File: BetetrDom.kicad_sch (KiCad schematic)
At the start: 10 parts, among them J1 XT60PW-M, J2 Raspberry_Pi_2_3

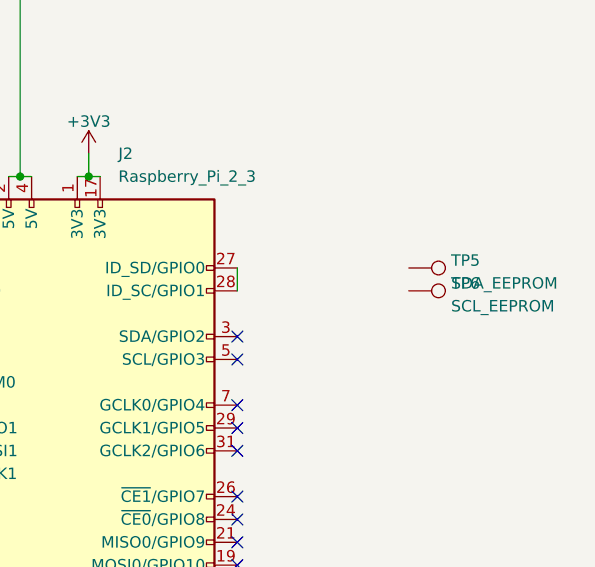
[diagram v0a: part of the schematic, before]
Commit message: UPDATE
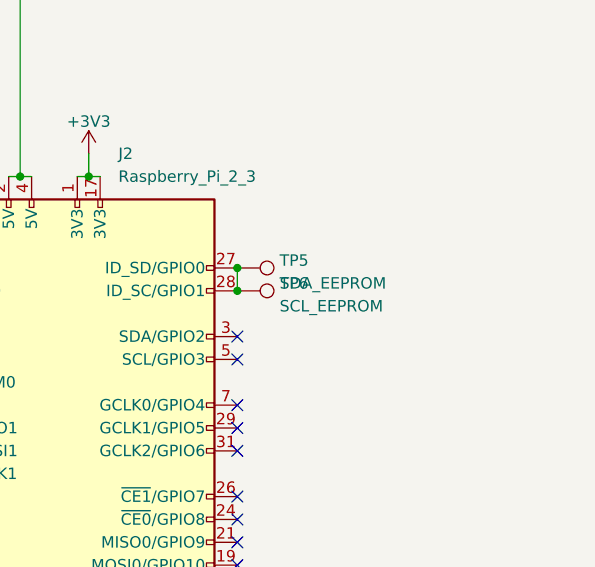
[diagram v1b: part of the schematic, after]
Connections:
- net at J2.27 (ID_SD/GPIO0), J2.28 (ID_SC/GPIO1): now also TP5.1, TP6.1
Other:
- moved on the sheet: TP5, TP6
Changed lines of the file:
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@@
 	(paper "A4")
+	(junction
+		(at 194.31 77.47)
+		(diameter 0)
+		(color 0 0 0 0)
+	)
 	(junction
 		(at 179.07 133.35)
@@
 	(junction
 		(at 41.91 59.69)
+		(diameter 0)
+		(color 0 0 0 0)
+	)
+	(junction
+		(at 194.31 80.01)
 		(diameter 0)
 		(color 0 0 0 0)
@@
 	(symbol
 		(lib_id "Connector:TestPoint")
-		(at 213.36 80.01 270)
+		(at 194.31 80.01 270)
 		(unit 1)
 		(exclude_from_sim no)
@@
 		(fields_autoplaced yes)
 		(property "Reference" "TP6"
-			(at 218.059 79.1753 90)
+			(at 199.009 79.1753 90)
 			(effects
 				(font
@@
 		)
 		(property "Value" "SCL_EEPROM"
-			(at 218.059 81.7122 90)
+			(at 199.009 81.7122 90)
 			(effects
 				(font
@@
 		)
 		(property "Footprint" "TestPoint:TestPoint_Pad_1.5x1.5mm"
-			(at 213.36 85.09 0)
+			(at 194.31 85.09 0)
 			(effects
 				(font
@@
 		)
 		(property "Datasheet" "~"
-			(at 213.36 85.09 0)
+			(at 194.31 85.09 0)
 			(effects
 				(font
@@
 		)
 		(property "Description" ""
-			(at 213.36 80.01 0)
+			(at 194.31 80.01 0)
 			(effects
 				(font
@@
 	(symbol
 		(lib_id "Connector:TestPoint")
-		(at 213.36 77.47 270)
+		(at 194.31 77.47 270)
 		(unit 1)
 		(exclude_from_sim no)
@@
 		(fields_autoplaced yes)
 		(property "Reference" "TP5"
-			(at 218.059 76.6353 90)
+			(at 199.009 76.6353 90)
 			(effects
 				(font
@@
 		)
 		(property "Value" "SDA_EEPROM"
-			(at 218.059 79.1722 90)
+			(at 199.009 79.1722 90)
 			(effects
 				(font
@@
 		)
 		(property "Footprint" "TestPoint:TestPoint_Pad_1.5x1.5mm"
-			(at 213.36 82.55 0)
+			(at 194.31 82.55 0)
 			(effects
 				(font
@@
 		)
 		(property "Datasheet" "~"
-			(at 213.36 82.55 0)
+			(at 194.31 82.55 0)
 			(effects
 				(font
@@
 		)
 		(property "Description" ""
-			(at 213.36 77.47 0)
-			(effects
-				(font
+			(at 194.31 77.47 0)
+			(effects
+				(font

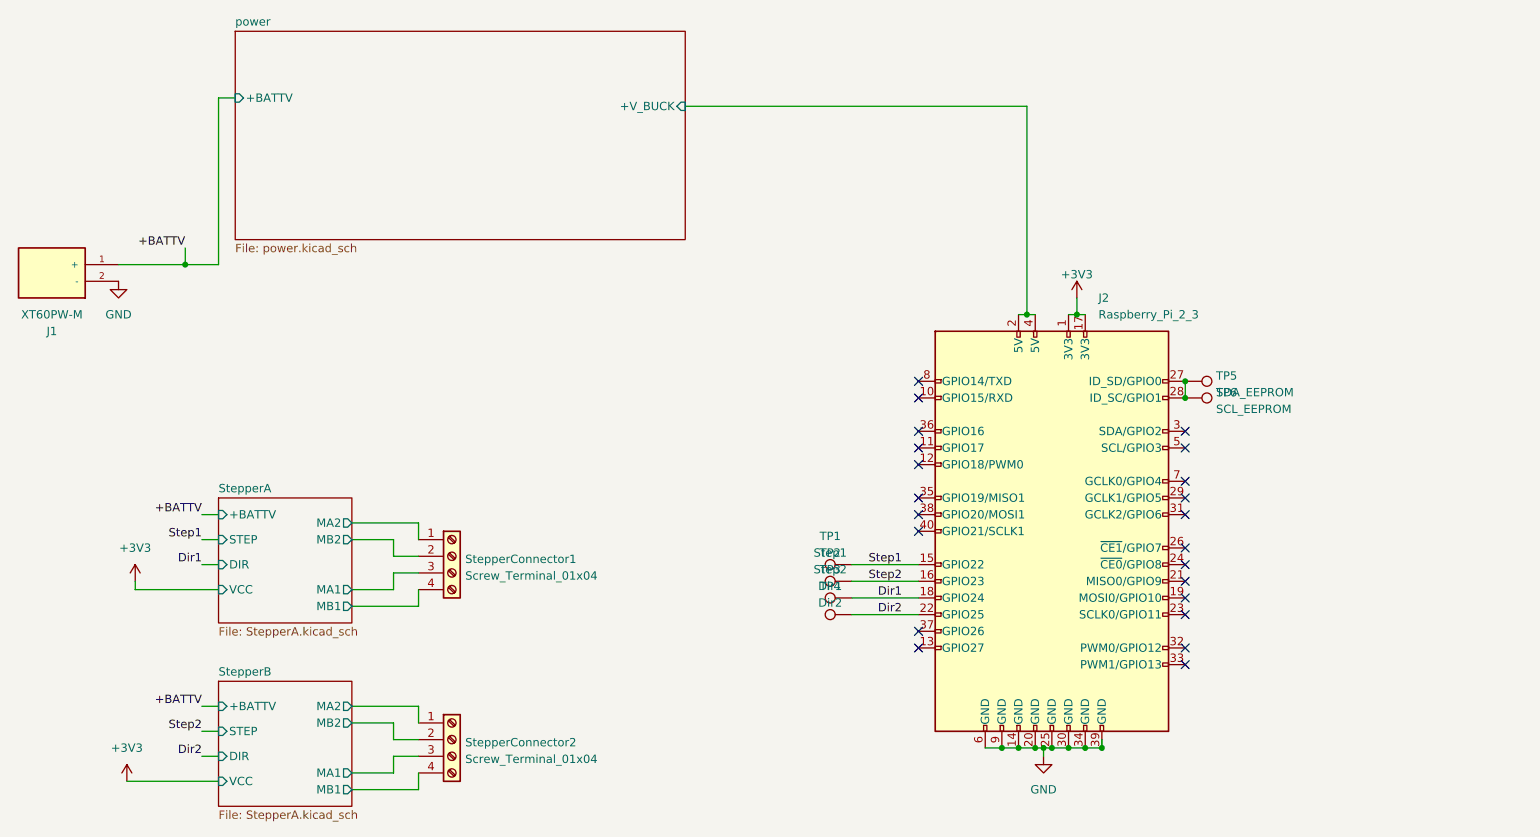
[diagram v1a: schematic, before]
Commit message: finished pcb layouts, ready for check p sure
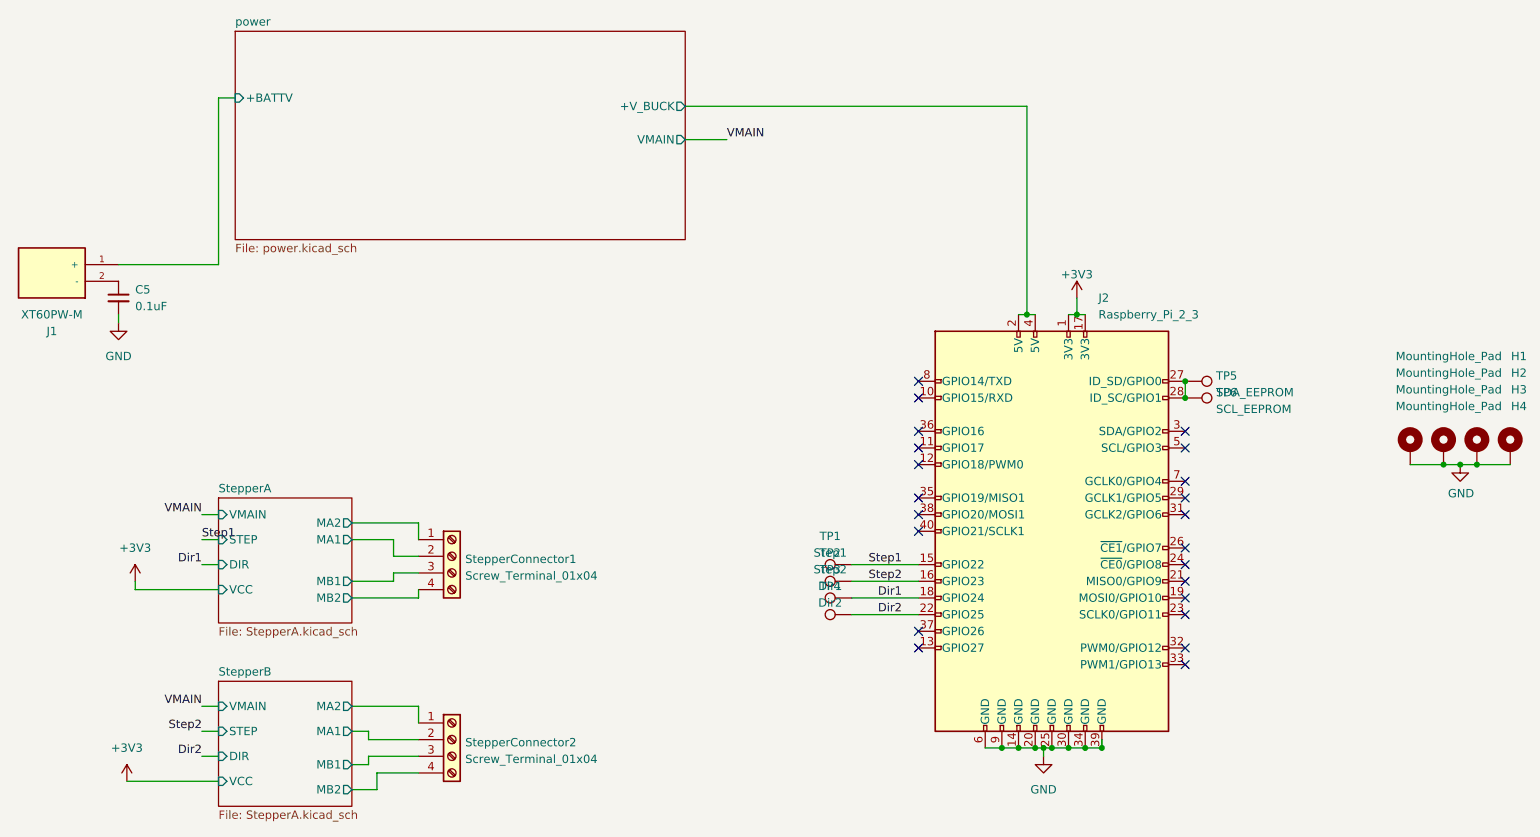
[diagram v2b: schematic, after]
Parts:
- added C5: 0.1uF, Capacitor_SMD:C_0402_1005Metric, symbol Device:C_Small
- added H1, H2, H3, H4: MountingHole_Pad, MountingHole:MountingHole_3.2mm_M3_DIN965_Pad, symbol Mechanical:MountingHole_Pad
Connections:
- net GND: now also C5.2, H1.1, H2.1, H3.1, H4.1; no longer J1.2 (-)
- net StepperA/MA1: now also StepperConnector1.2 (Pin_2); no longer StepperConnector1.3 (Pin_3)
- net StepperA/MB1: now also StepperConnector1.3 (Pin_3); no longer StepperConnector1.4 (Pin_4)
- net StepperA/MB2: now also StepperConnector1.4 (Pin_4); no longer StepperConnector1.2 (Pin_2)
- net StepperB/MA1: now also StepperConnector2.2 (Pin_2); no longer StepperConnector2.3 (Pin_3)
- net StepperB/MB1: now also StepperConnector2.3 (Pin_3); no longer StepperConnector2.4 (Pin_4)
- net StepperB/MB2: now also StepperConnector2.4 (Pin_4); no longer StepperConnector2.2 (Pin_2)
- net +BATTV renamed power/+BATTV
- new net: C5.1, J1.2 (-)
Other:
- sheet StepperA ports: added VMAIN; removed +BATTV
- sheet StepperB ports: added VMAIN; removed +BATTV
- sheet power ports: added VMAIN; removed none

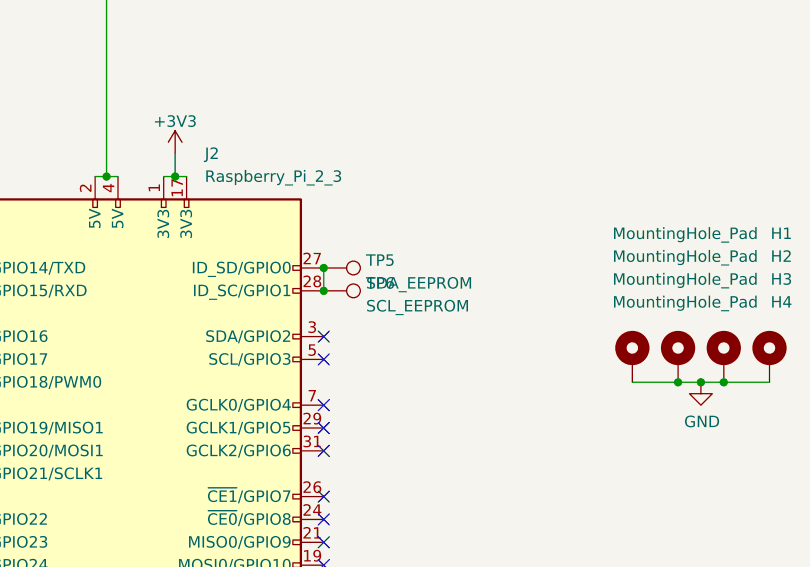
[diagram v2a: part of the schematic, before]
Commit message: update
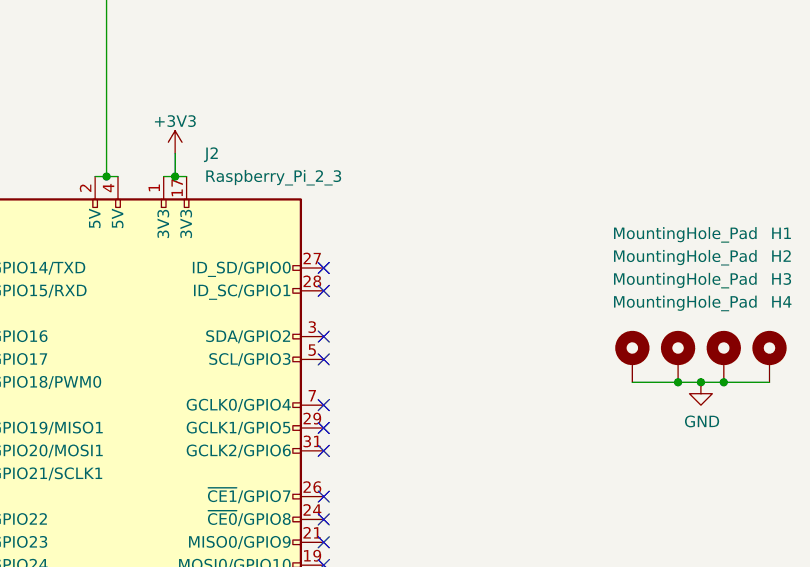
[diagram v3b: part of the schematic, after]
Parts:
- removed TP5: SDA_EEPROM, TestPoint:TestPoint_Pad_1.5x1.5mm, symbol Connector:TestPoint
- removed TP6: SCL_EEPROM, TestPoint:TestPoint_Pad_1.5x1.5mm, symbol Connector:TestPoint
- StepperConnector1, StepperConnector2: footprint TerminalBlock_TE-Connectivity:TerminalBlock_TE_282834-4_1x04_P2.54mm_Horizontal -> Connector_Molex:Molex_Nano-Fit_105313-xx04_1x04_P2.50mm_Horizontal
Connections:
- net at J2.27 (ID_SD/GPIO0): no longer J2.28 (ID_SC/GPIO1)
- no-connect marks 22 -> 24
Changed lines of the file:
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@@
 	(paper "A4")
-	(junction
-		(at 194.31 77.47)
-		(diameter 0)
-		(color 0 0 0 0)
-	)
 	(junction
 		(at 233.68 90.17)
@@
 	)
 	(junction
-		(at 194.31 80.01)
-		(diameter 0)
-		(color 0 0 0 0)
-	)
-	(junction
 		(at 166.37 133.35)
 		(diameter 0)
@@
 	)
 	(no_connect
+		(at 194.31 80.01)
+	)
+	(no_connect
+		(at 194.31 77.47)
+	)
+	(no_connect
 		(at 194.31 92.71)
 	)
@@
 		(pts
 			(xy 69.85 130.81) (xy 67.31 130.81)
-		)
-		(stroke
-			(width 0)
-			(type default)
-		)
-	)
-	(wire
-		(pts
-			(xy 194.31 77.47) (xy 194.31 80.01)
 		)
 		(stroke
@@
 	)
 	(symbol
-		(lib_id "Connector:TestPoint")
-		(at 194.31 80.01 270)
-		(unit 1)
-		(exclude_from_sim no)
-		(in_bom yes)
-		(on_board yes)
-		(dnp no)
-		(fields_autoplaced yes)
-		(property "Reference" "TP6"
-			(at 199.009 79.1753 90)
-			(effects
-				(font
-					(size 1.27 1.27)
-				)
-				(justify left)
-			)
-		)
-		(property "Value" "SCL_EEPROM"
-			(at 199.009 81.7122 90)
-			(effects
-				(font
-					(size 1.27 1.27)
-				)
-				(justify left)
-			)
-		)
-		(property "Footprint" "TestPoint:TestPoint_Pad_1.5x1.5mm"
-			(at 194.31 85.09 0)
-			(effects
-				(font
-					(size 1.27 1.27)
-				)
-				(hide yes)
-			)
-		)
-		(property "Datasheet" "~"
-			(at 194.31 85.09 0)
-			(effects
-				(font
-					(size 1.27 1.27)
-				)
-				(hide yes)
-			)
-		)
-		(property "Description" ""
-			(at 194.31 80.01 0)
-			(effects
-				(font
-					(size 1.27 1.27)
-				)
-				(hide yes)
-			)
-		)
-		(pin "1"
-		)
-		(instances
-			(project "BetetrDom"
-				(path "/3d73b00f-865e-402b-88ef-ae22e0a8ba36"
-					(reference "TP6")
-					(unit 1)
-				)
-			)
-		)
-	)
-	(symbol
 		(lib_id "Connector:Screw_Terminal_01x04")
 		(at 82.55 104.14 0)
@@
 			)
 		)
-		(property "Footprint" "TerminalBlock_TE-Connectivity:TerminalBlock_TE_282834-4_1x04_P2.54mm_Horizontal"
+		(property "Footprint" "Connector_Molex:Molex_Nano-Fit_105313-xx04_1x04_P2.50mm_Horizontal"
 			(at 82.55 104.14 0)
 			(effects
@@
 			)
 		)
-		(property "Footprint" "TerminalBlock_TE-Connectivity:TerminalBlock_TE_282834-4_1x04_P2.54mm_Horizontal"
+		(property "Footprint" "Connector_Molex:Molex_Nano-Fit_105313-xx04_1x04_P2.50mm_Horizontal"
 			(at 82.55 132.08 0)
 			(effects
@@
 					(unit 1)
 				)
-			)
-		)
-	)
-	(symbol
-		(lib_id "Connector:TestPoint")
-		(at 194.31 77.47 270)
-		(unit 1)
-		(exclude_from_sim no)
-		(in_bom yes)
-		(on_board yes)
-		(dnp no)
-		(fields_autoplaced yes)
-		(property "Reference" "TP5"
-			(at 199.009 76.6353 90)
-			(effects
-				(font
-					(size 1.27 1.27)
-				)
-				(justify left)
-			)
-		)
-		(property "Value" "SDA_EEPROM"
-			(at 199.009 79.1722 90)
-			(effects
-				(font
-					(size 1.27 1.27)
-				)
-				(justify left)
-			)
-		)
-		(property "Footprint" "TestPoint:TestPoint_Pad_1.5x1.5mm"
-			(at 194.31 82.55 0)
-			(effects
-				(font
-					(size 1.27 1.27)
-				)
-				(hide yes)
-			)
-		)
-		(property "Datasheet" "~"
-			(at 194.31 82.55 0)
-			(effects
-				(font
-					(size 1.27 1.27)
-				)
-				(hide yes)
-			)
-		)
-		(property "Description" ""
-			(at 194.31 77.47 0)
-			(effects
-				(font
-					(size 1.27 1.27)
-				)
-				(hide yes)
-			)
-		)
-		(pin "1"
-		)
-		(instances
-			(project "BetetrDom"
-				(path "/3d73b00f-865e-402b-88ef-ae22e0a8ba36"
-					(reference "TP5")
-					(unit 1)
-				)
